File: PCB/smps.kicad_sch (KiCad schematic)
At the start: 10 parts, among them U2 LM2576S-ADJ

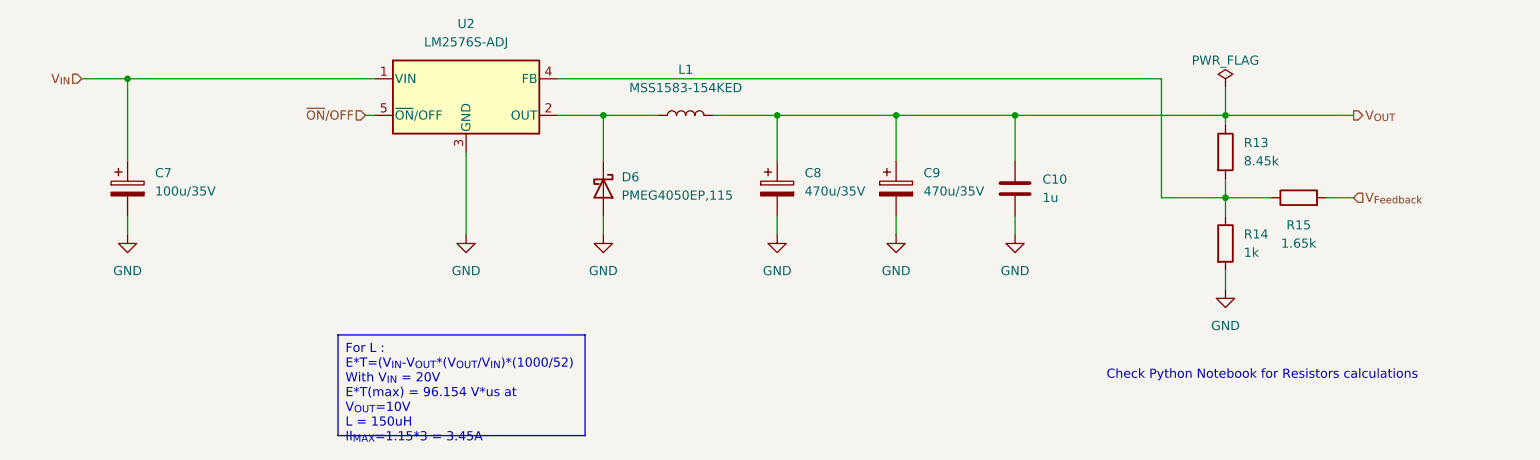
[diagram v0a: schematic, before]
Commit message: ok for dcdc and cleanup
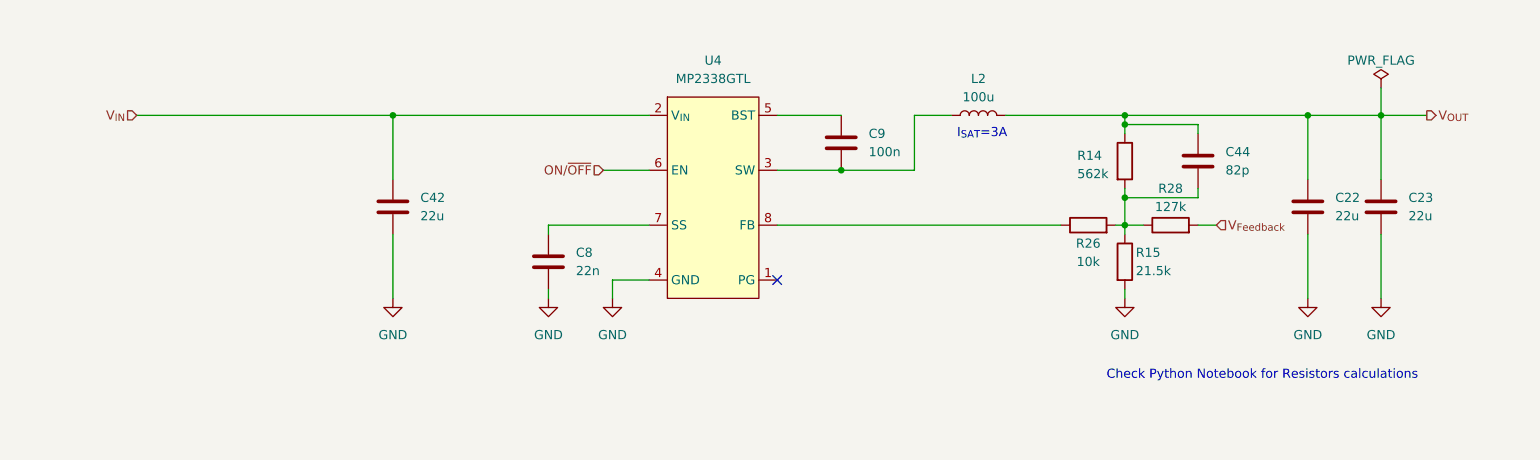
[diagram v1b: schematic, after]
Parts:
- removed C10: 1u, Capacitor_SMD:C_0603_1608Metric, symbol Device:C
- removed C7: 100u/35V, Capacitor_SMD:CP_Elec_6.3x7.7, symbol Device:C_Polarized
- removed C8, C9: 470u/35V, Capacitor_SMD:CP_Elec_8x10, symbol Device:C_Polarized
- removed D6: PMEG4050EP,115, Diode_SMD:D_SOD-128, symbol Device:D_Schottky
- removed L1: MSS1583-154KED, TattooSupplyFootprints:MSS1583, symbol Device:L
- removed R13: 8.45k, Resistor_SMD:R_0603_1608Metric, symbol Device:R
- removed U2: LM2576S-ADJ, Package_TO_SOT_SMD:TO-263-5_TabPin3, symbol Regulator_Switching:LM2576S-ADJ
- added C22, C23, C42: 22u, symbol Device:C
- added C44: 82p, symbol Device:C
- added C8: 22n, symbol Device:C
- added C9: 100n, symbol Device:C
- added L2: 100u, symbol Device:L
- added R26: 10k, symbol Device:R
- added R28: 127k, symbol Device:R
- added U4: MP2338GTL, Package_TO_SOT_SMD:SOT-583-8, symbol TattooSupplyLib:MP2338GTL
- R14: value 1k -> 562k; footprint Resistor_SMD:R_0603_1608Metric -> (none); MPN ERJ-3EKF1001V -> (none); Manufacturer Panasonic -> (none)
- R15: value 1.65k -> 21.5k; footprint Resistor_SMD:R_0603_1608Metric -> (none); MPN ERJ-3EKF1651V -> (none); Manufacturer Panasonic -> (none)
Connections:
- net GND: now also R15.2, C22.2, C23.2, C42.2, C8.2, U4.4 (GND); no longer R14.2
- net V_{Feedback}: now also R28.2; no longer R15.2
- net V_{IN}: now also C42.1, U4.2 (V_{IN})
- net V_{OUT}: now also R14.1, C22.1, C23.1, C44.1, L2.2
- net at R15.1: now also R14.2, C44.2, R26.2, R28.1; no longer R14.1
- new net: C8.1, U4.7 (SS)
- new net: C9.2, L2.1, U4.3 (SW)
- new net: C9.1, U4.5 (BST)
- new net: R26.1, U4.8 (FB)
- new net ON/~{OFF}: U4.6 (EN)
- no-connect marks 0 -> 1
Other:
- note added: "I_{SAT}=3A"
